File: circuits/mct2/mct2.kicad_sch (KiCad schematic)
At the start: 17 parts

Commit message: Aug 31, 2024
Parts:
- J?: footprint (none) -> Connector_PinHeader_2.54mm:PinHeader_1x02_P2.54mm_Vertical
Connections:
- net USB_CAM_N: now also A1.84 (USB2_P8-); no longer A1.114 (USB2_P6-)
- net USB_CAM_P: now also A1.82 (USB2_P8+); no longer A1.112 (USB2_P6+)
- net USB_M2E_N: now also A1.78 (USB2_P7-); no longer A1.109 (USB2_P5-)
- net USB_M2E_P: now also A1.76 (USB2_P7+); no longer A1.111 (USB2_P5+)
- net USB_SMEC_N: now also A1.109 (USB2_P5-); no longer A1.78 (USB2_P7-)
- net USB_SMEC_P: now also A1.111 (USB2_P5+); no longer A1.76 (USB2_P7+)
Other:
- note added: "July 4, 2024 - August 31, 2024"
- note removed: "July 4, 2024 - August 11, 2024"
- moved on the sheet: A1, BT?, C?, J?, R?, SW?, U?

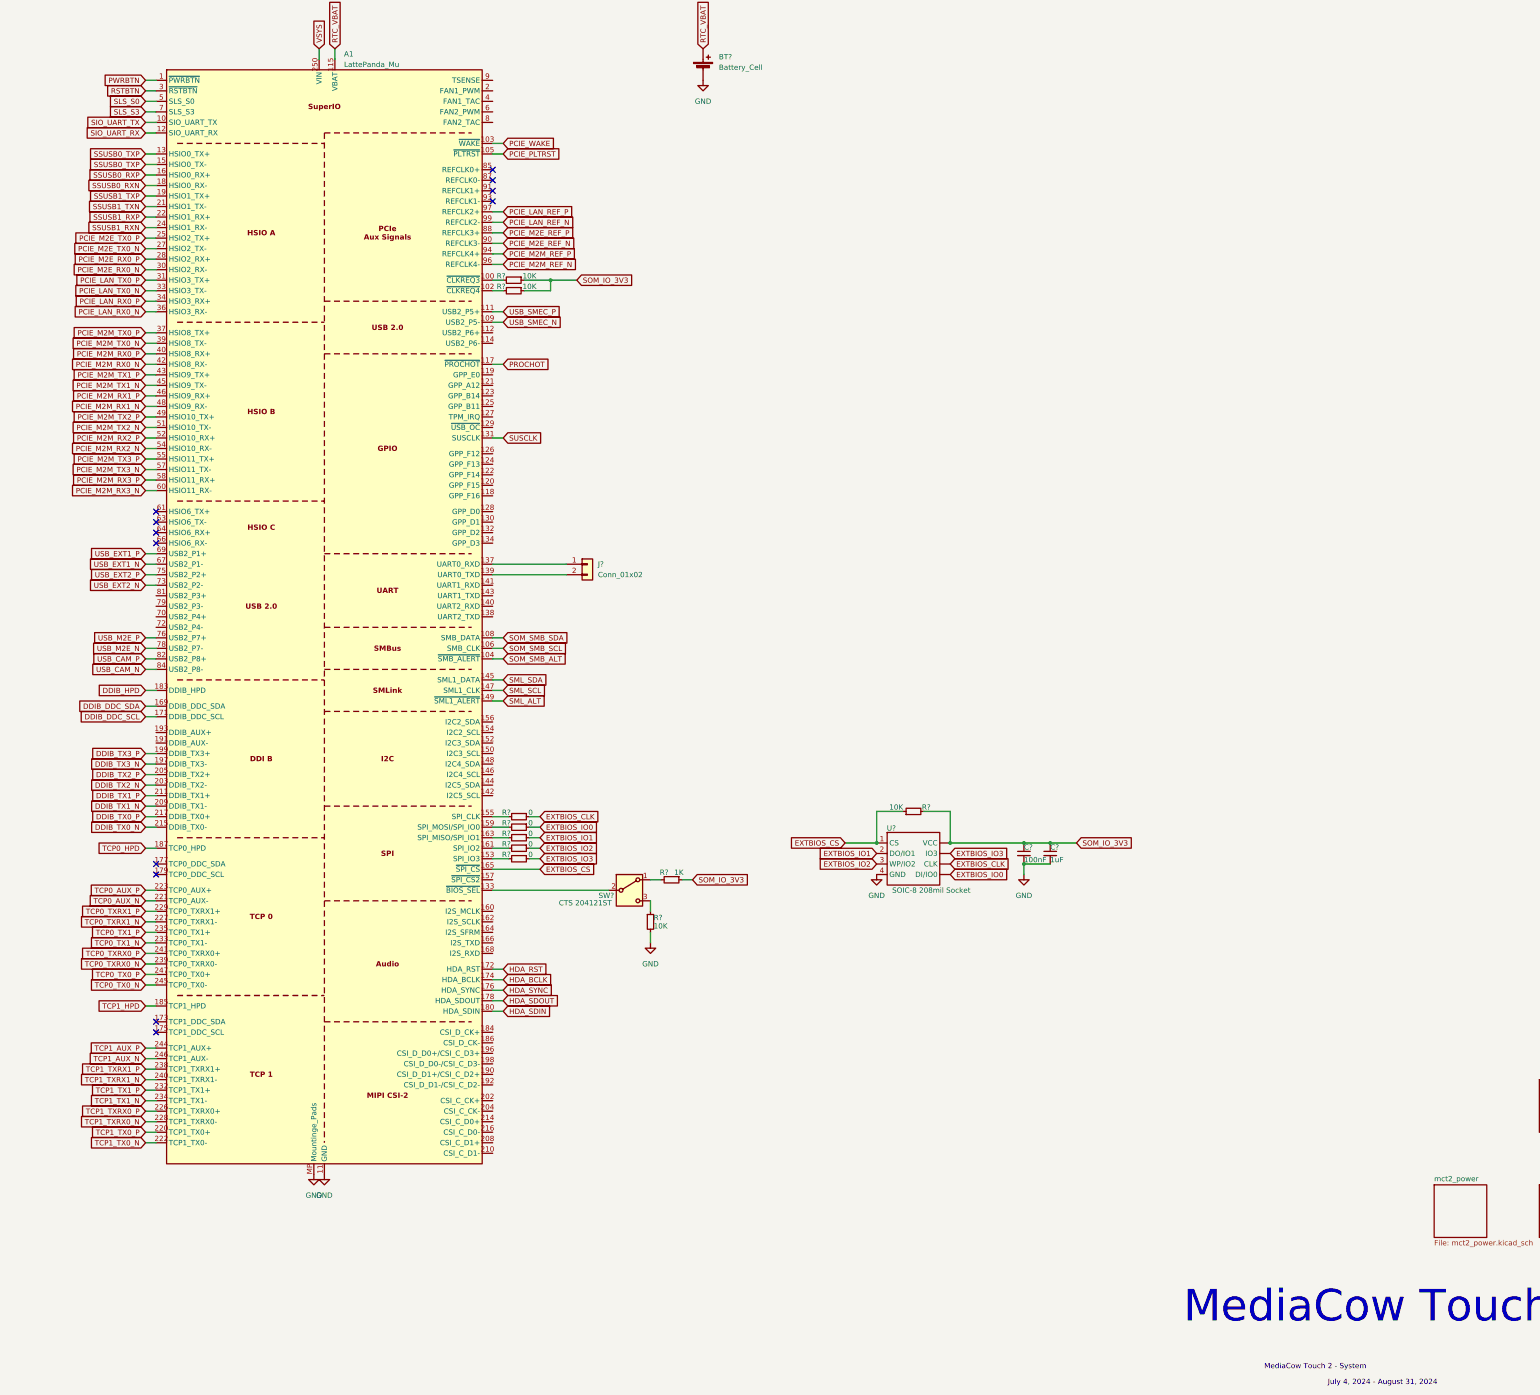
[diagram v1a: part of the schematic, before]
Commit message: Sep 4, 2024 1
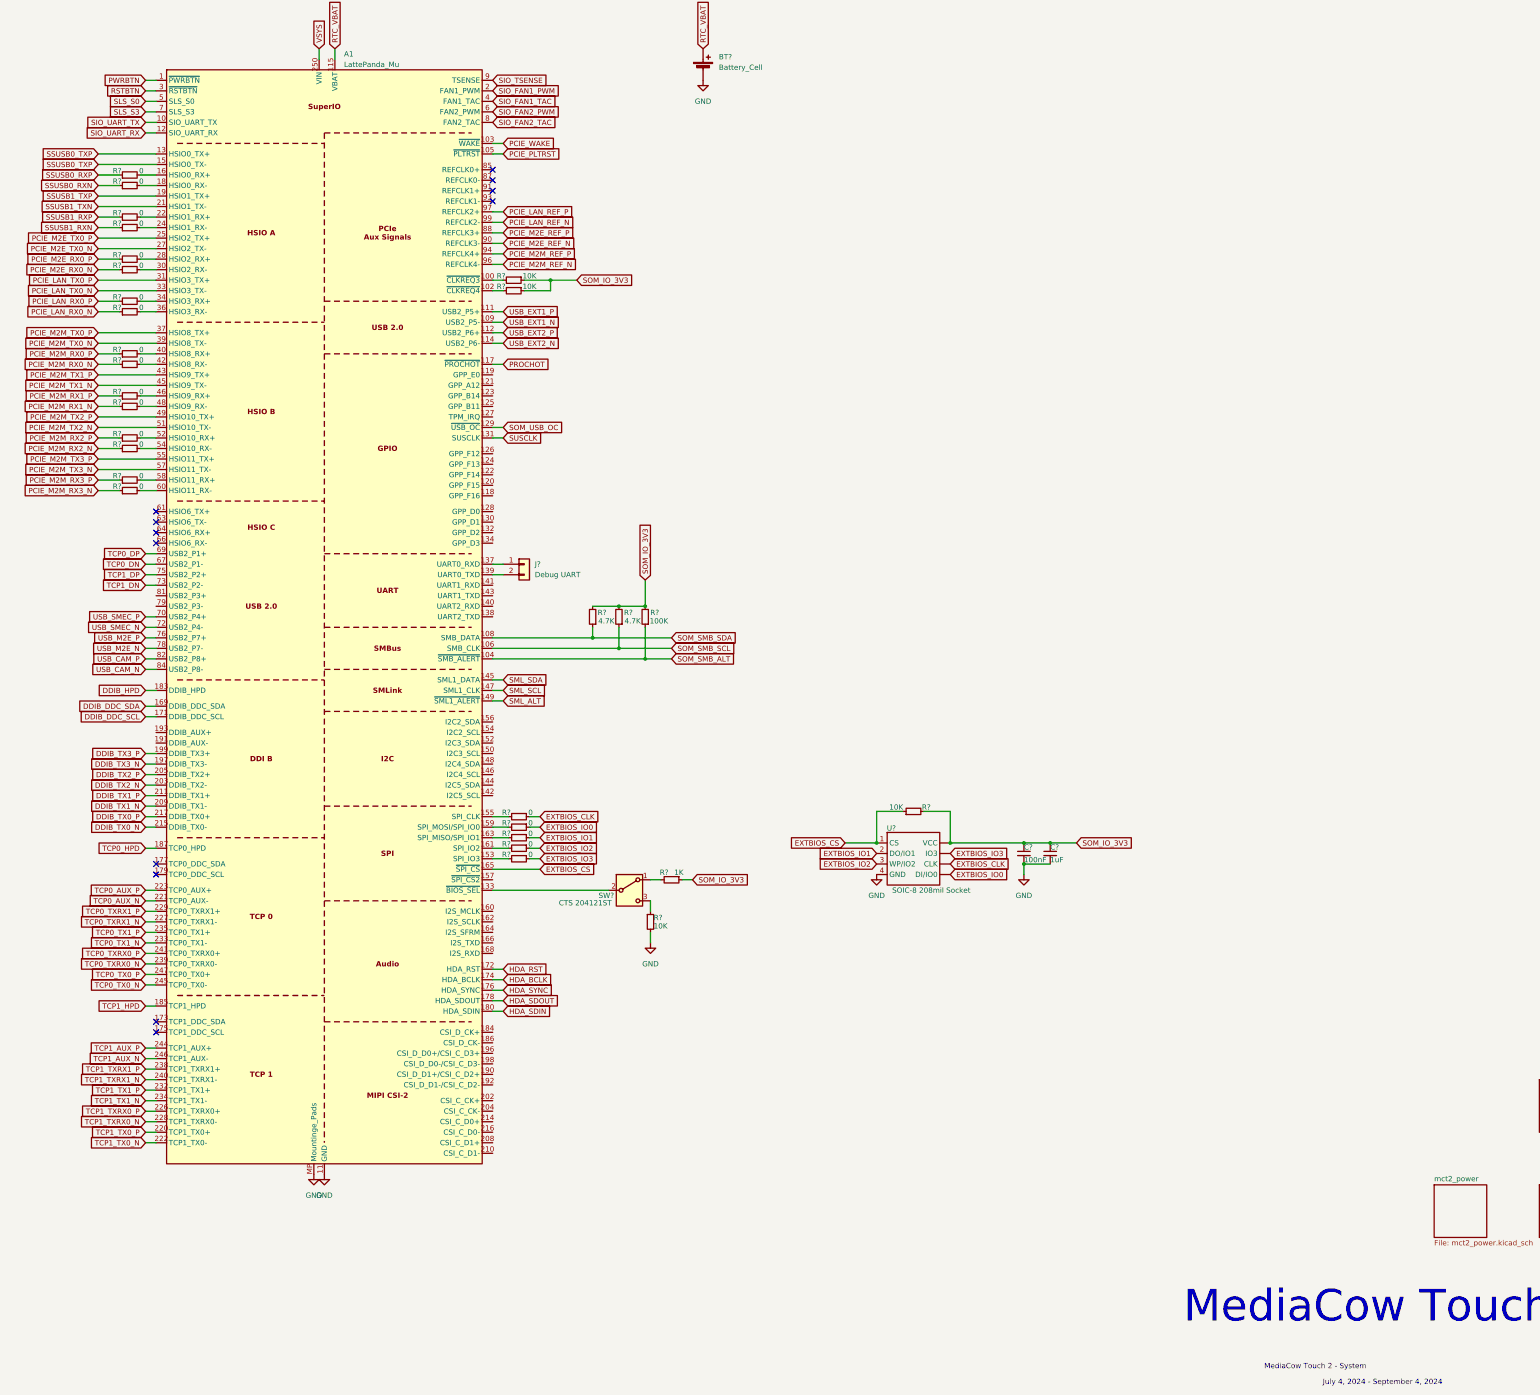
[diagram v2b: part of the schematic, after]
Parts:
- added R? (x16): 0, Resistor_SMD:R_0402_1005Metric, symbol Device:R_Small
- added R?: 100K, symbol Device:R_Small
- added R? (x2): 4.7K, symbol Device:R_Small
- J?: value Conn_01x02 -> Debug UART
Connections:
- net PCIE_LAN_RX0_N: now also R?.1; no longer A1.36 (HSIO3_RX-)
- net PCIE_LAN_RX0_P: now also R?.1; no longer A1.34 (HSIO3_RX+)
- net PCIE_M2E_RX0_N: now also R?.1; no longer A1.30 (HSIO2_RX-)
- net PCIE_M2E_RX0_P: now also R?.1; no longer A1.28 (HSIO2_RX+)
- net PCIE_M2M_RX0_N: now also R?.1; no longer A1.42 (HSIO8_RX-)
- net PCIE_M2M_RX0_P: now also R?.1; no longer A1.40 (HSIO8_RX+)
- net PCIE_M2M_RX1_N: now also R?.1; no longer A1.48 (HSIO9_RX-)
- net PCIE_M2M_RX1_P: now also R?.1; no longer A1.46 (HSIO9_RX+)
- net PCIE_M2M_RX2_N: now also R?.1; no longer A1.54 (HSIO10_RX-)
- net PCIE_M2M_RX2_P: now also R?.1; no longer A1.52 (HSIO10_RX+)
- net PCIE_M2M_RX3_N: now also R?.1; no longer A1.60 (HSIO11_RX-)
- net PCIE_M2M_RX3_P: now also R?.1; no longer A1.58 (HSIO11_RX+)
- net SOM_IO_3V3: now also R?.2, R?.2, R?.2
- net SOM_SMB_ALT: now also R?.1
- net SOM_SMB_SCL: now also R?.1
- net SOM_SMB_SDA: now also R?.1
- net SSUSB0_RXN: now also R?.1; no longer A1.18 (HSIO0_RX-)
- net SSUSB0_RXP: now also R?.1; no longer A1.16 (HSIO0_RX+)
- net SSUSB1_RXN: now also R?.1; no longer A1.24 (HSIO1_RX-)
- net SSUSB1_RXP: now also R?.1; no longer A1.22 (HSIO1_RX+)
- net USB_EXT1_N: now also A1.109 (USB2_P5-); no longer A1.67 (USB2_P1-)
- net USB_EXT1_P: now also A1.111 (USB2_P5+); no longer A1.69 (USB2_P1+)
- net USB_EXT2_N: now also A1.114 (USB2_P6-); no longer A1.73 (USB2_P2-)
- net USB_EXT2_P: now also A1.112 (USB2_P6+); no longer A1.75 (USB2_P2+)
- net USB_SMEC_N: now also A1.72 (USB2_P4-); no longer A1.109 (USB2_P5-)
- net USB_SMEC_P: now also A1.70 (USB2_P4+); no longer A1.111 (USB2_P5+)
- net SOM_USB_OC: now reaches A1.129 (~{USB_OC})
- net SIO_FAN1_PWM: now reaches A1.2 (FAN1_PWM)
- net SIO_FAN1_TAC: now reaches A1.4 (FAN1_TAC)
- net SIO_FAN2_PWM: now reaches A1.6 (FAN2_PWM)
- net SIO_FAN2_TAC: now reaches A1.8 (FAN2_TAC)
- net SIO_TSENSE: now reaches A1.9 (TSENSE)
- new net: A1.58 (HSIO11_RX+), R?.2
- new net: A1.16 (HSIO0_RX+), R?.2
- new net: A1.30 (HSIO2_RX-), R?.2
- new net: A1.34 (HSIO3_RX+), R?.2
- new net: A1.42 (HSIO8_RX-), R?.2
- new net: A1.28 (HSIO2_RX+), R?.2
- new net: A1.46 (HSIO9_RX+), R?.2
- new net: A1.52 (HSIO10_RX+), R?.2
- new net: A1.48 (HSIO9_RX-), R?.2
- new net: A1.36 (HSIO3_RX-), R?.2
- new net: A1.22 (HSIO1_RX+), R?.2
- new net: A1.24 (HSIO1_RX-), R?.2
- new net: A1.18 (HSIO0_RX-), R?.2
- new net: A1.40 (HSIO8_RX+), R?.2
- new net: A1.54 (HSIO10_RX-), R?.2
- new net: A1.60 (HSIO11_RX-), R?.2
- new net TCP0_DN: A1.67 (USB2_P1-)
- new net TCP0_DP: A1.69 (USB2_P1+)
- new net TCP1_DN: A1.73 (USB2_P2-)
- new net TCP1_DP: A1.75 (USB2_P2+)
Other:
- note added: "July 4, 2024 - September 4, 2024"
- note removed: "July 4, 2024 - August 31, 2024"
- moved on the sheet: J?
